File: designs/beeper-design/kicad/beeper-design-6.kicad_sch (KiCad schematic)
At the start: 24 parts, among them U13 CSD75207W15, U3 BQ51003YFPR, U5 FH19C-6S-0.5SH(10)

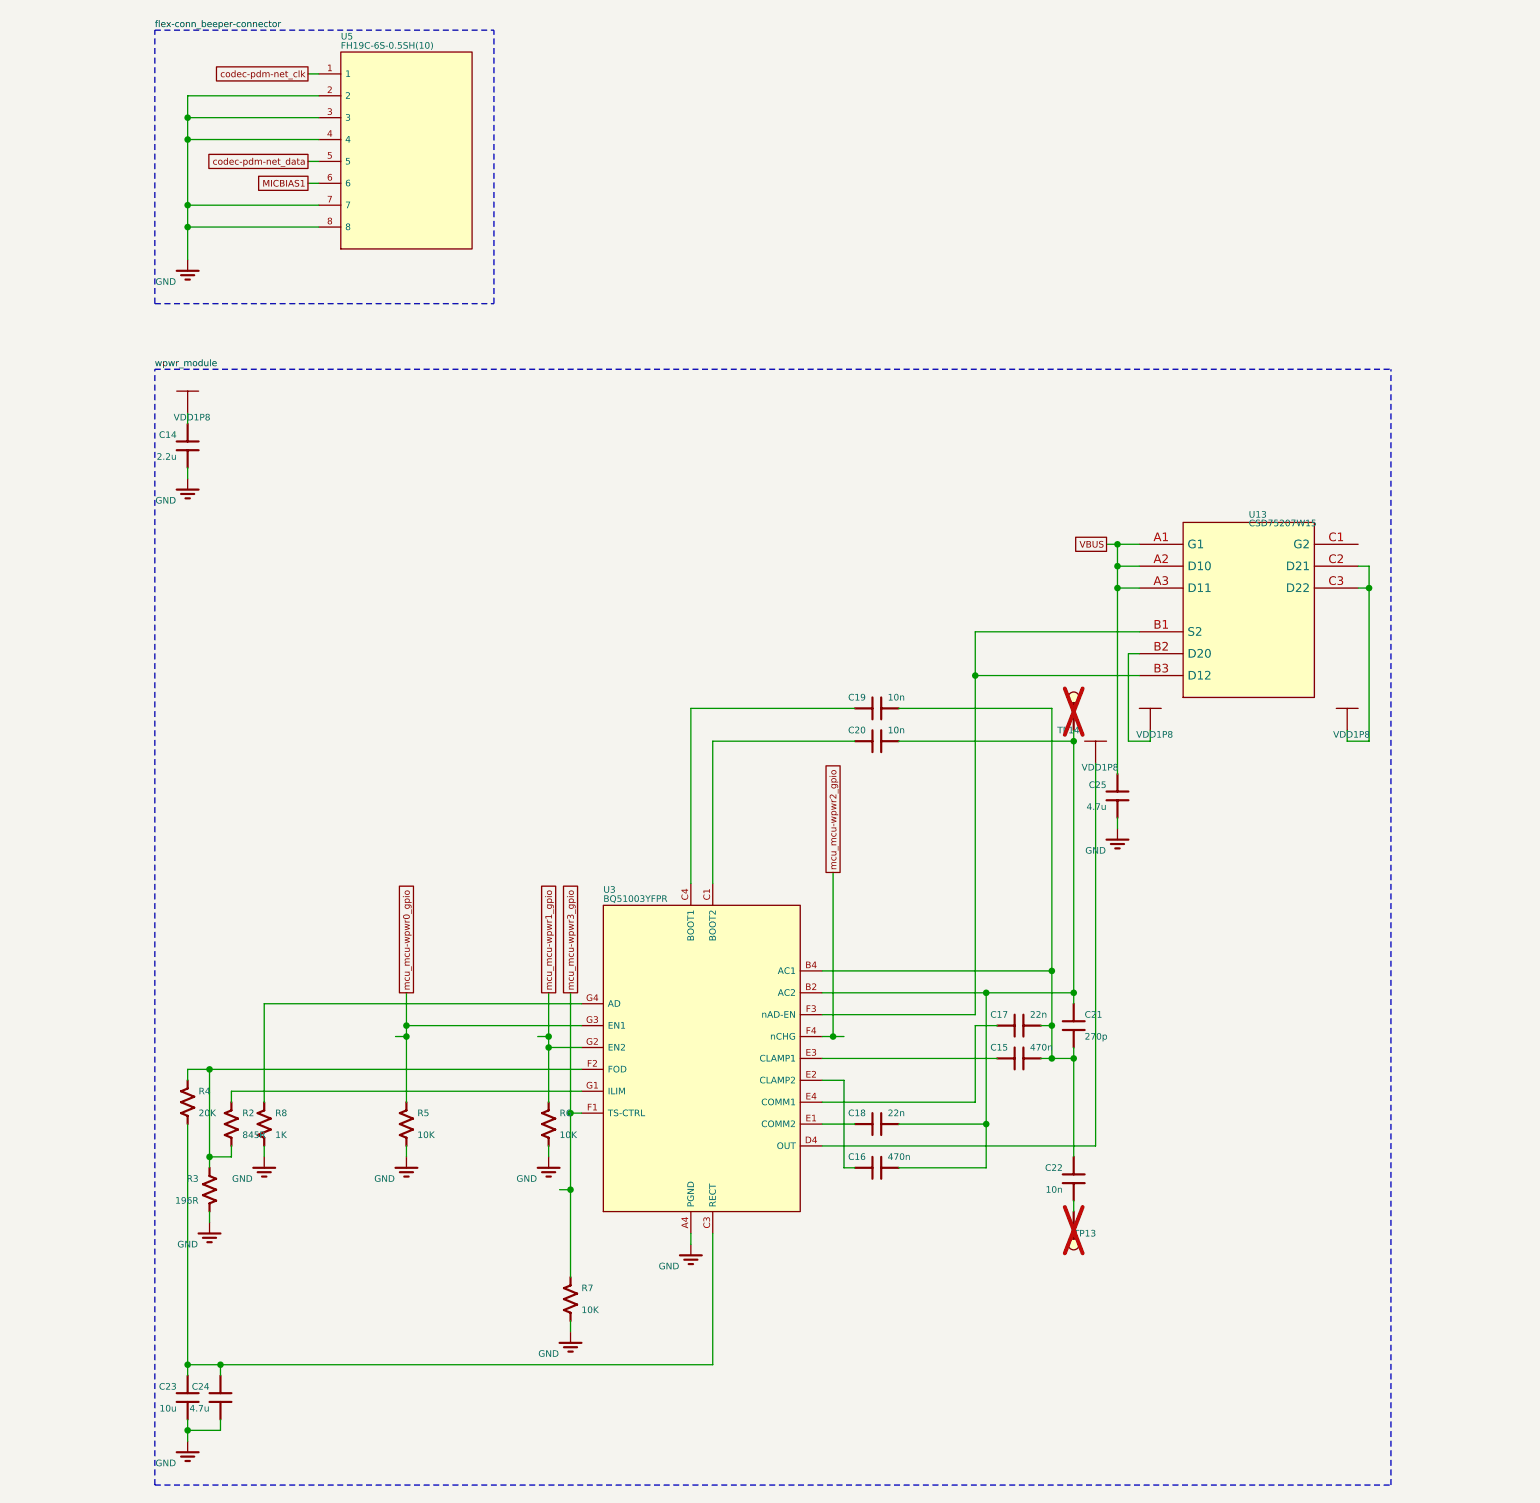
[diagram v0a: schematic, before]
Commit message: another export
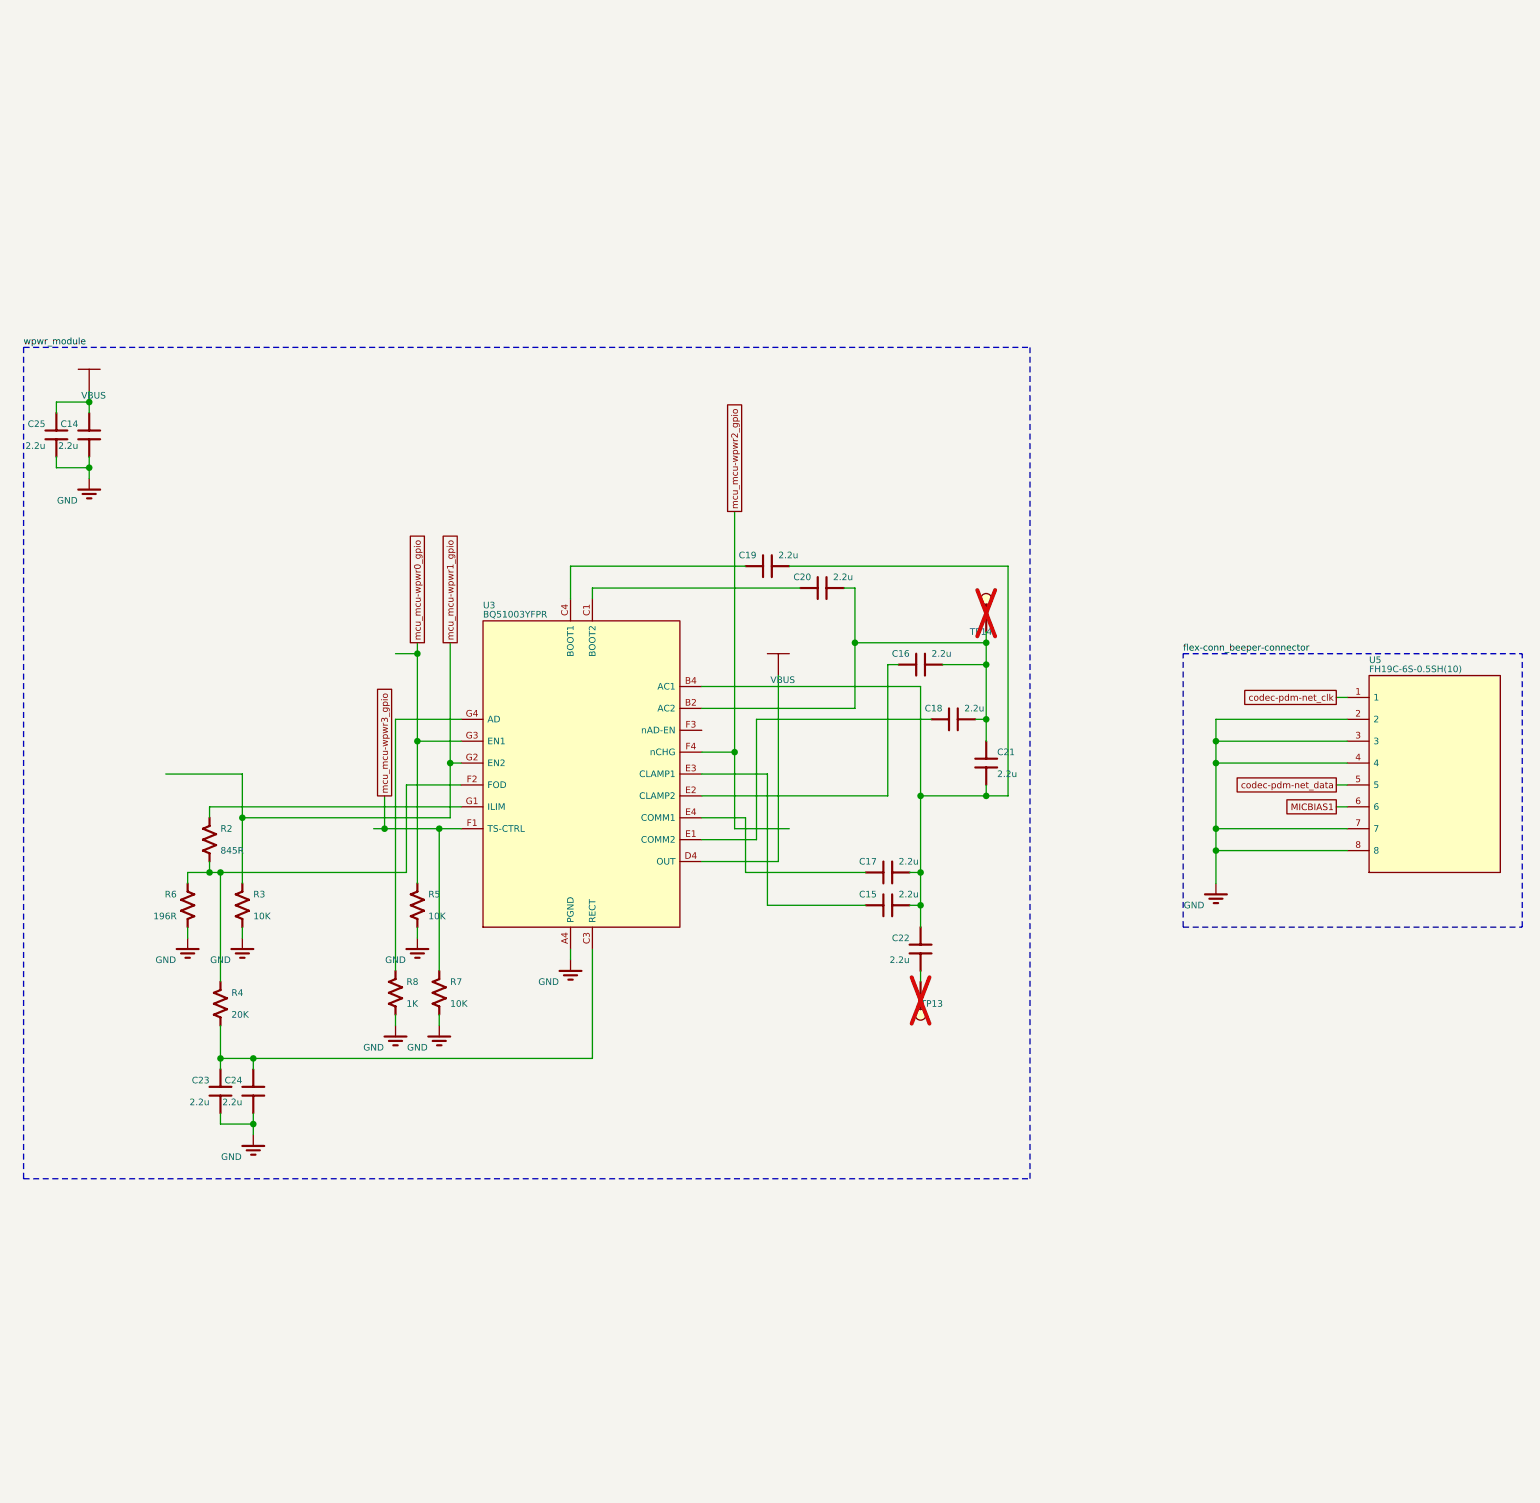
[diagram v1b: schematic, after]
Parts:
- removed C14: 2.2u, beeper-design:Pkg0201_25, symbol my_capacitor_7
- removed C15: 470n, beeper-design:Pkg0201_21, symbol my_capacitor_5
- removed C16: 470n, beeper-design:Pkg0201_31, symbol my_capacitor_10
- removed C17: 22n, beeper-design:Pkg0201_45, symbol my_capacitor_18
- removed C18: 22n, beeper-design:Pkg0201_9, symbol my_capacitor_2
- removed C19: 10n, beeper-design:Pkg0201_18, symbol my_capacitor_4
- removed C20: 10n, beeper-design:Pkg0201_30, symbol my_capacitor_9
- removed C21: 270p, beeper-design:Pkg0201_43, symbol my_capacitor_16
- removed C22: 10n, beeper-design:Pkg0201_7, symbol my_capacitor
- removed C23: 10u, beeper-design:Pkg0402_2, symbol C105225_2
- removed C24: 4.7u, beeper-design:Pkg0402_6, symbol C23733_1
- removed C25: 4.7u, beeper-design:Pkg0402_4, symbol C23733
- removed R2: 845R, beeper-design:Pkg0201_36, symbol my_resistor_10
- removed R3: 196R, beeper-design:Pkg0201_2, symbol C138167
- removed R4: 20K, beeper-design:Pkg0201_12, symbol my_resistor_3
- removed R5: 10K, beeper-design:Pkg0201_22, symbol my_resistor_7
- removed R6: 10K, beeper-design:Pkg0201_34, symbol my_resistor_9
- removed R7: 10K, beeper-design:Pkg0201, symbol my_resistor_12
- removed R8: 1K, beeper-design:Pkg0201_11, symbol my_resistor_2
- removed U13: CSD75207W15, beeper-design:LP_6, symbol CSD75207W15
- added C14: 2.2u, beeper-design:Pkg0201_2, symbol C335106
- added C15: 2.2u, beeper-design:Pkg0201_51, symbol C335106_35
- added C16: 2.2u, beeper-design:Pkg0201_12, symbol C335106_10
- added C17: 2.2u, beeper-design:Pkg0201_25, symbol C335106_18
- added C18: 2.2u, beeper-design:Pkg0201_37, symbol C335106_26
- added C19: 2.2u, beeper-design:Pkg0201_49, symbol C335106_33
- added C20: 2.2u, beeper-design:Pkg0201_10, symbol C335106_8
- added C21: 2.2u, beeper-design:Pkg0201_23, symbol C335106_16
- added C22: 2.2u, beeper-design:Pkg0201_35, symbol C335106_25
- added C23: 2.2u, beeper-design:Pkg0201_48, symbol C335106_32
- added C24: 2.2u, beeper-design:Pkg0201_7, symbol C335106_5
- added C25: 2.2u, beeper-design:Pkg0201_22, symbol C335106_15
- added R2: 845R, beeper-design:Pkg0201_15, symbol my_resistor_1
- added R3: 10K, beeper-design:Pkg0201_14, symbol my_resistor
- added R4: 20K, beeper-design:Pkg0201_41, symbol my_resistor_10
- added R5: 10K, beeper-design:Pkg0201, symbol my_resistor_14
- added R6: 196R, beeper-design:Pkg0201_28, symbol C138167
- added R7: 10K, beeper-design:Pkg0201_26, symbol my_resistor_5
- added R8: 1K, beeper-design:Pkg0201_38, symbol my_resistor_8
- U3: footprint beeper-design:LP_7 -> beeper-design:LP_6
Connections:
- net VDD1P8 is gone; now on net VBUS: U3.D1 (OUT), U3.D2 (OUT), U3.D3 (OUT), U3.D4 (OUT)
- net GND: now also C14.1, C23.1, C24.1, C25.1, R3.2, R5.2, R6.2, R7.2, R8.2
- net VBUS: now also C14.2, C25.2
- net mcu_mcu-wpwr0_gpio: now also R5.1
- net mcu_mcu-wpwr1_gpio: now also R3.1
- net mcu_mcu-wpwr3_gpio: now also R7.1
- net at U3.B3 (AC1), U3.B4 (AC1): now also C15.1, C17.1, C19.1, C21.2, C22.2
- net at U3.C4 (BOOT1): now also C19.2
- net at TP14.p, U3.B1 (AC2), U3.B2 (AC2): now also C16.1, C18.1, C20.1, C21.1
- net at U3.C1 (BOOT2): now also C20.2
- net at U3.C2 (RECT), U3.C3 (RECT): now also C23.2, C24.2, R4.2
- net at U3.G1 (ILIM): now also R2.1
- net at U3.F2 (FOD): now also R2.2, R4.1, R6.1
- net at U3.E3 (CLAMP1): now also C15.2
- net at U3.E1 (COMM2): now also C18.2
- net at U3.E2 (CLAMP2): now also C16.2
- net at U3.E4 (COMM1): now also C17.2
- net at U3.G4 (AD): now also R8.1
- net at TP13.p: now also C22.1
